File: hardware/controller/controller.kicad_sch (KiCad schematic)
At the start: 45 parts, among them J1 USB_C_Receptacle_PowerOnly_6P, J2 Bat, SW1 SW_SPST, SW2 RKJXV1224005, SW3 RKJXV1224005, SW4 TC-1102N-C-AS-B, SW5 TS-1199A-B-B, SW6 TC-1102N-C-AS-B, SW7 SK-12D07-L3-B, SW8 TS-1199A-B-B, U1 TP4059, U3 AMS1117, U4 ESP32-C3-WROOM-02-N4

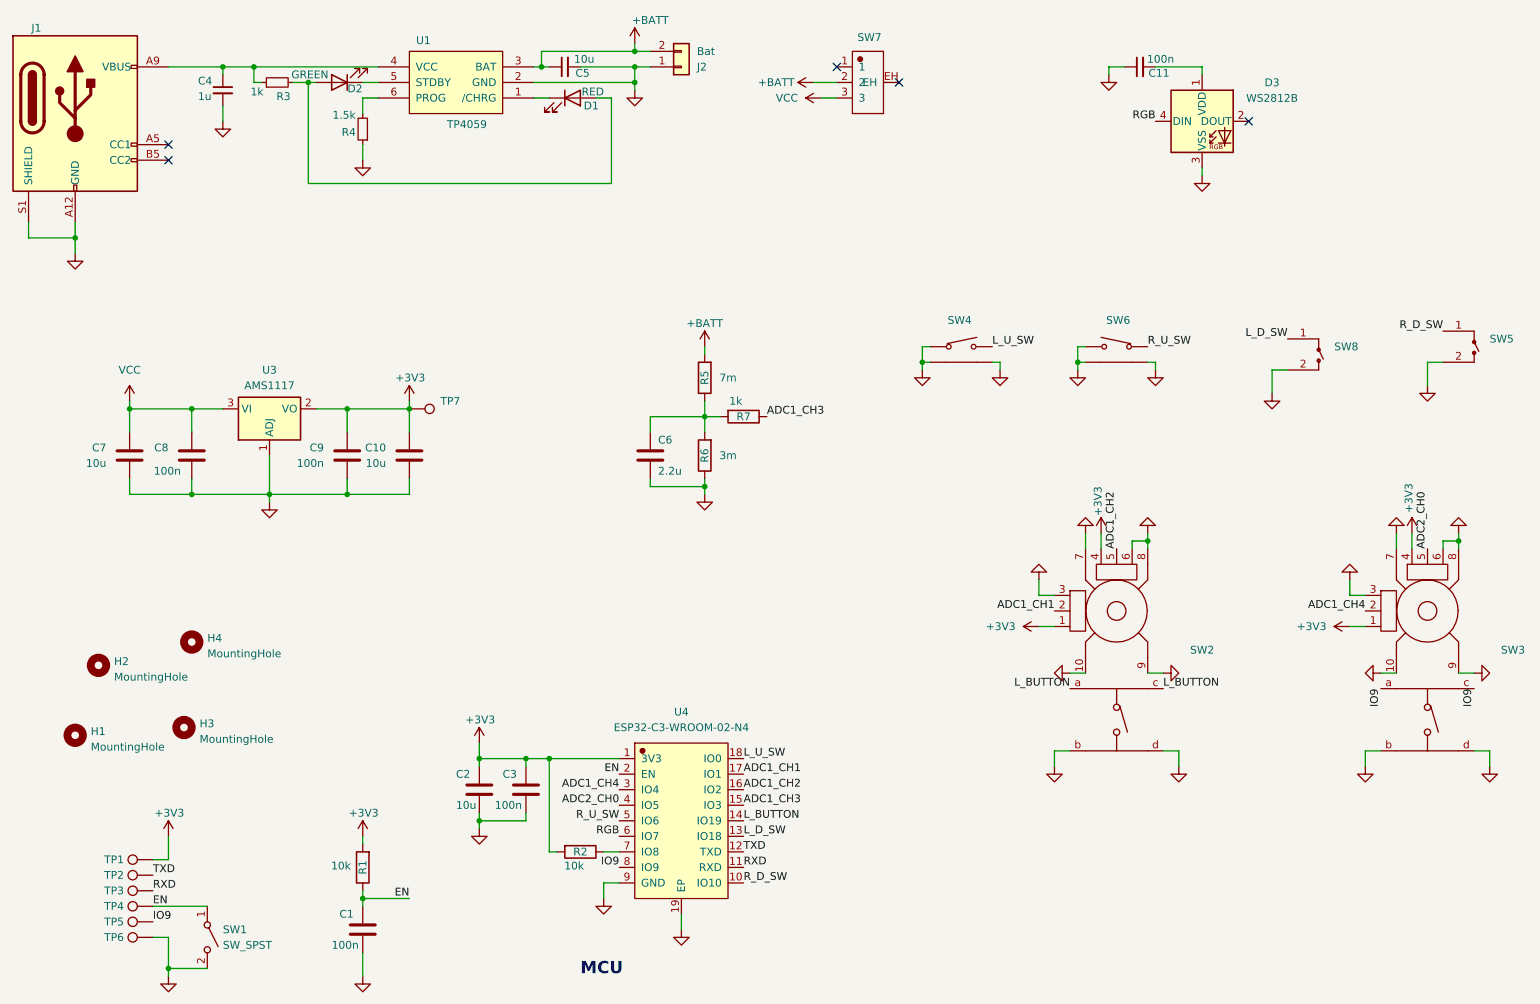
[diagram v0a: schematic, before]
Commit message: update rfBat pcb
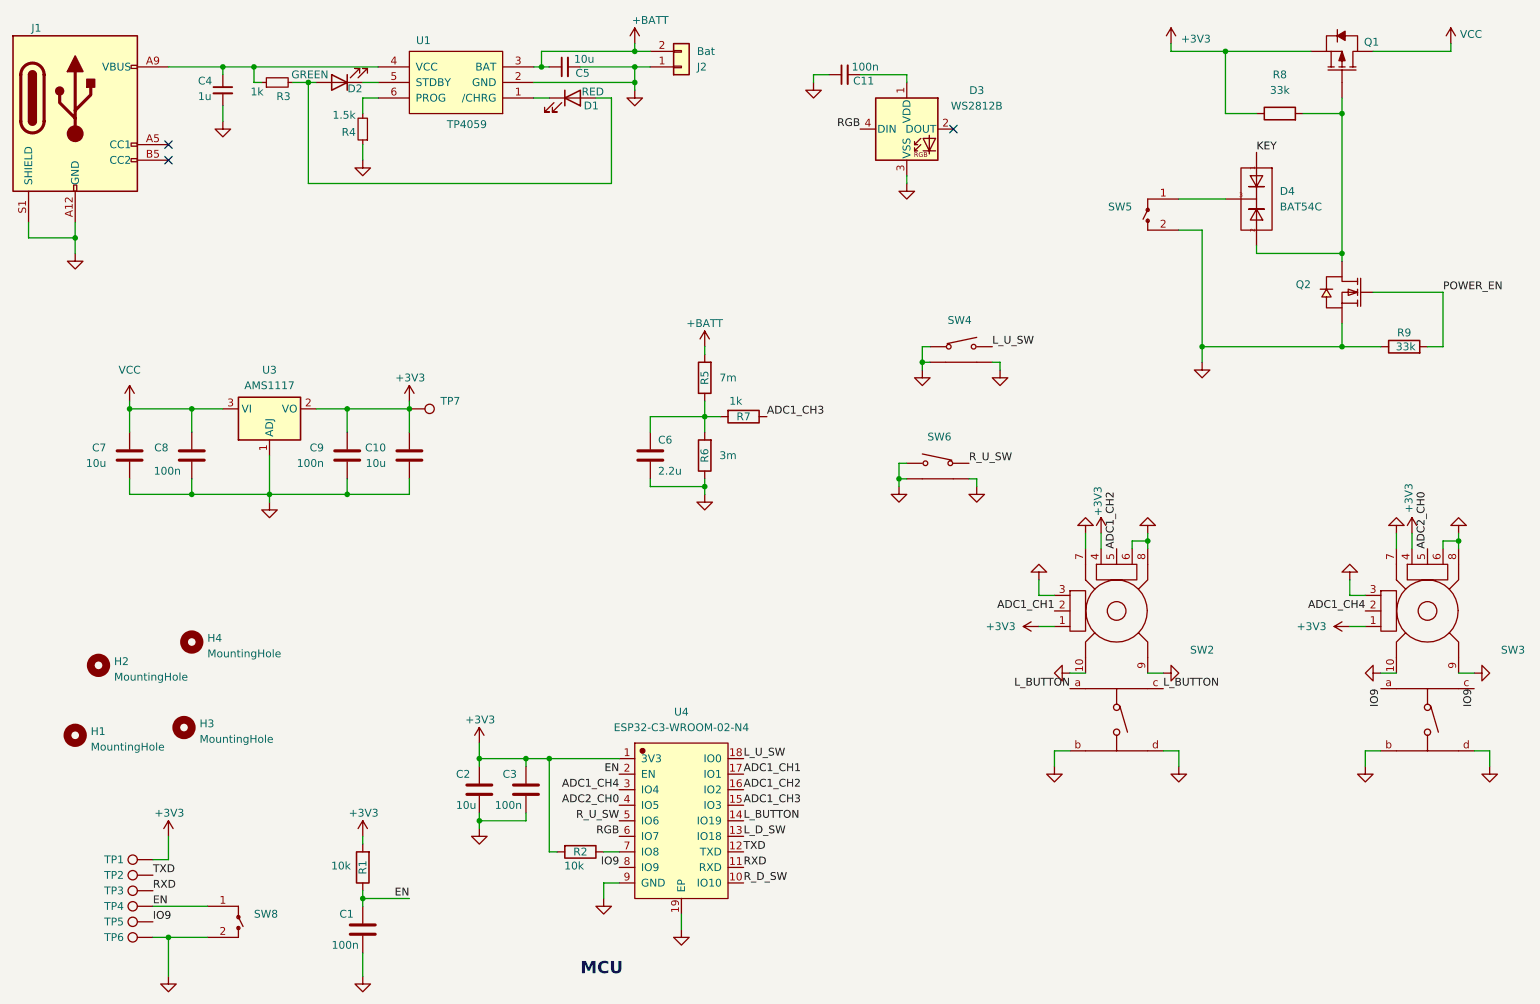
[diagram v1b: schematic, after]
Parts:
- removed SW1: SW_SPST, Button_Switch_SMD:SW_SPST_B3U-1000P, symbol Switch:SW_SPST
- removed SW7: SK-12D07-L3-B, Button_Switch_SMD:SW_SPDT_CK_JS102011SAQN, symbol espController:SK-12D07-L3-B
- added D4: BAT54C, bat_rf:BAT54C, symbol bat_rf:BAT54C
- added Q1: AO3401, bat_rf:AO3401, symbol bat_rf:AO3401
- added Q2: AllPower__AP2300, bat_rf:SOT-23, symbol bat_rf:AllPower__AP2300
- added R8, R9: 33k, Resistor_SMD:R_0603_1608Metric_Pad0.98x0.95mm_HandSolder, symbol Device:R
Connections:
- net +3V3: now also Q1.2 (S), R8.1
- net EN: now also SW8.1
- net GND: now also Q2.2 (S), R9.1
- net L_D_SW: no longer SW8.1
- net R_D_SW: no longer SW5.1
- net VCC: now also Q1.3 (D)
- new net: D4.3 (C), SW5.1
- new net: D4.2 (A), Q1.1 (G), Q2.3 (D), R8.2
- new net KEY: D4.1 (A)
- new net POWER_EN: Q2.1 (G), R9.2
- no-connect marks 5 -> 3
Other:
- moved on the sheet: C11, D3, SW5, SW6, SW8
